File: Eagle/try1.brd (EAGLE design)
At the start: 35.2 x 47 mm, 7 parts, among them M1 WIRELESS-NRF24L01

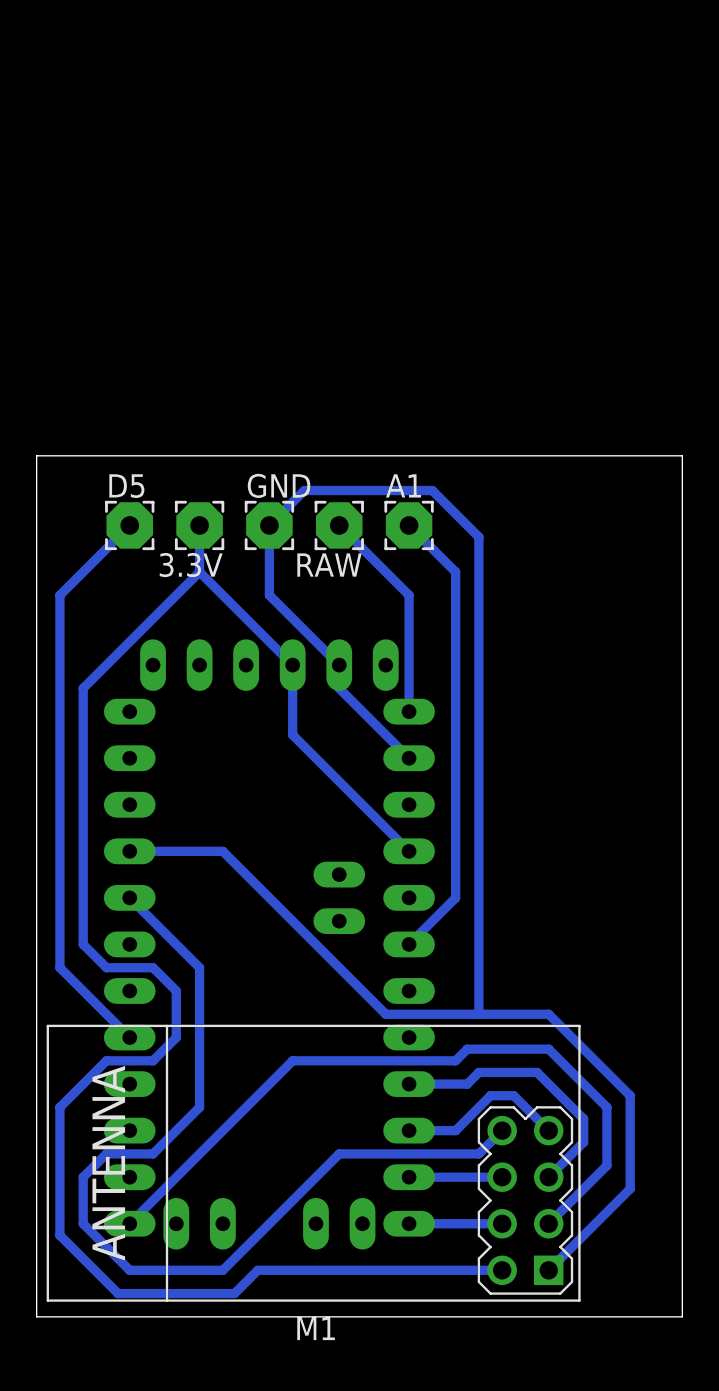
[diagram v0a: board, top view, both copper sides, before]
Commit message: Just cleaning up and updating the eagle files.
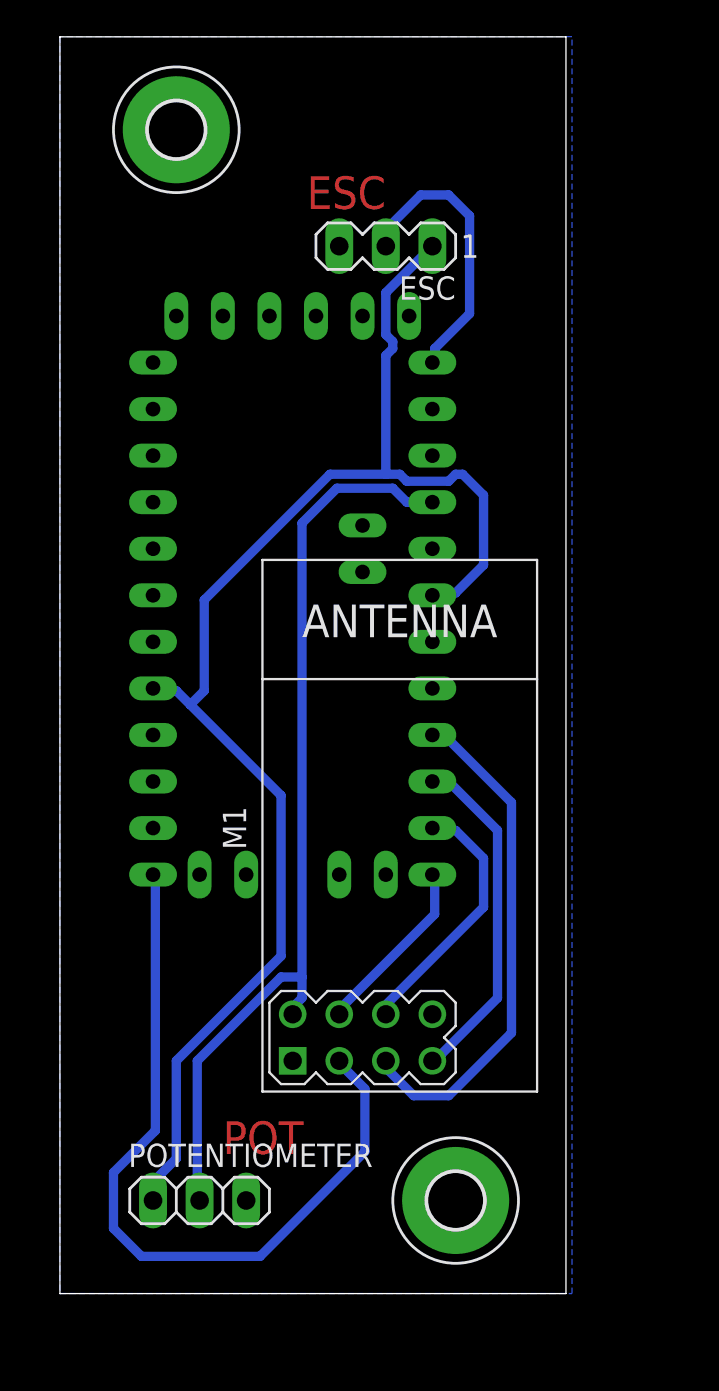
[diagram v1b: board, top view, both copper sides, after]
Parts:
- removed 3.3V, A1, D5, GND, RAW: (no value), wirepad:2,54/1,0
- added ESC: (no value), con-lstb:MA03-1
- added H1, H2: MOUNT-PAD-ROUND3.0, holes:3,0-PAD
- added POTENTIOMETER: (no value), pinhead:1X03
- moved U$2 19.1 mm to (15.2, 36.8)
- moved M1 18.5 mm to (20.3, 24.1), turned to 90 degrees
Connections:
- removed net IRQ: M1.8, U$2.D2
- removed net N$1: D5.1, U$2.D5
- removed net N$2: A1.1, U$2.A1
- removed net N$3: RAW.1, U$2.RAW
- new net RAW: ESC.2, U$2.RAW
- new net SIG: ESC.1, POTENTIOMETER.1, U$2.A1, U$2.D5
- net GND: now also ESC.3, POTENTIOMETER.3; no longer GND.1, U$2.GND2
- net VCC: now also POTENTIOMETER.2; no longer 3.3V.1, U$2.VCC1
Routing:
- net GND: track 99.4 -> 0.00 mm
- net SIG: track 0.00 -> 80.5 mm
- net IRQ: track 50.5 -> 0.00 mm
- net VCC: track 95.0 -> 50.8 mm
- net N$1: track 31.1 -> 0.00 mm
- net N$2: track 25.0 -> 0.00 mm
- net RAW: track 0.00 -> 15.6 mm
- net SCK: track 14.8 -> 27.8 mm
- net N$3: track 11.7 -> 0.00 mm
- net MISO: track 9.20 -> 19.3 mm
- net MOSI: track 5.08 -> 15.0 mm
- net CSN: track 5.08 -> 9.91 mm
- net CE: track 39.0 -> 42.7 mm
- added copper zone on layer 16, net GND
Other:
- board size 35.2 x 47 mm -> 27.6 x 68.6 mm
- board text added: "ESC"
- board text added: "POT"
